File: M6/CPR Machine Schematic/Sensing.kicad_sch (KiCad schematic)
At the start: 14 parts, among them J6 I2C Port, J9 Force Sensor, U4 MCP6004, U5 MCP3021A5T-E_OT

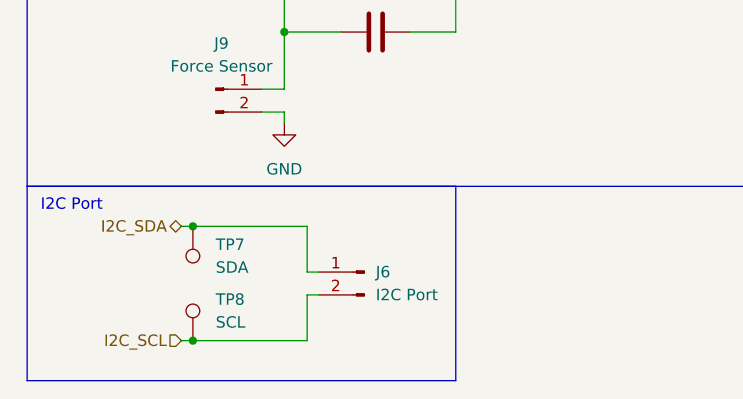
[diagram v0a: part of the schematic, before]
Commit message: More Revisions
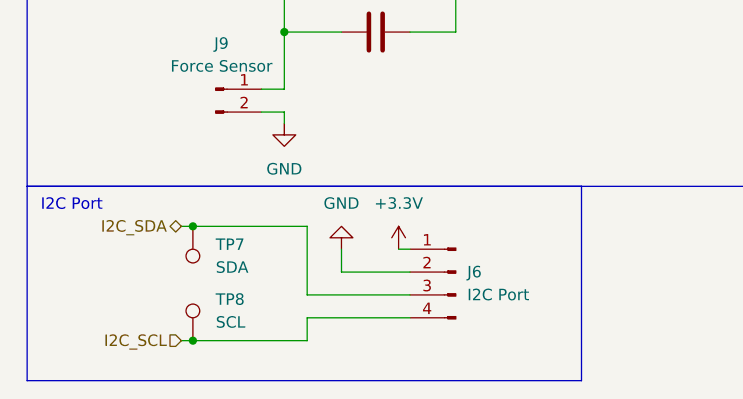
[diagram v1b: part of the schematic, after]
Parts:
- J6: footprint Connector_PinHeader_2.54mm:PinHeader_1x02_P2.54mm_Vertical -> Connector_PinHeader_2.54mm:PinHeader_1x04_P2.54mm_Vertical; symbol Connector:Conn_01x02_Pin -> Connector:Conn_01x04_Pin; now in the parts list
- U5: footprint 2679:IC_MCP3021A5T-E_OT -> 2679:IC_MCP3021A0T-E_OT
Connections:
- net +3.3V: now also J6.1 (Pin_1)
- net GND: now also J6.2 (Pin_2)
- net I2C_SCL: now also J6.4 (Pin_4); no longer J6.2 (Pin_2)
- net I2C_SDA: now also J6.3 (Pin_3); no longer J6.1 (Pin_1)
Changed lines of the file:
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@@
 	(rectangle
 		(start 14.605 84.455)
-		(end 62.23 106.045)
+		(end 76.2 106.045)
 		(stroke
 			(width 0)
@@
 	(wire
 		(pts
+			(xy 55.88 91.44) (xy 57.15 91.44)
+		)
+		(stroke
+			(width 0)
+			(type default)
+		)
+	)
+	(wire
+		(pts
 			(xy 33.02 101.6) (xy 31.75 101.6)
 		)
@@
 	(wire
 		(pts
-			(xy 45.72 93.98) (xy 46.99 93.98)
+			(xy 45.72 96.52) (xy 57.15 96.52)
+		)
+		(stroke
+			(width 0)
+			(type default)
+		)
+	)
+	(wire
+		(pts
+			(xy 49.53 91.44) (xy 49.53 93.98)
 		)
 		(stroke
@@
 	(wire
 		(pts
-			(xy 45.72 88.9) (xy 45.72 93.98)
+			(xy 45.72 88.9) (xy 45.72 96.52)
 		)
 		(stroke
@@
 	(wire
 		(pts
-			(xy 45.72 96.52) (xy 45.72 101.6)
+			(xy 45.72 99.06) (xy 45.72 101.6)
 		)
 		(stroke
@@
 	(wire
 		(pts
-			(xy 45.72 96.52) (xy 46.99 96.52)
+			(xy 45.72 99.06) (xy 57.15 99.06)
 		)
 		(stroke
@@
 		(pts
 			(xy 43.18 77.47) (xy 43.18 76.2)
+		)
+		(stroke
+			(width 0)
+			(type default)
+		)
+	)
+	(wire
+		(pts
+			(xy 49.53 93.98) (xy 57.15 93.98)
 		)
 		(stroke
@@
 	)
 	(symbol
-		(lib_id "Connector:Conn_01x02_Pin")
-		(at 52.07 93.98 0)
+		(lib_id "Connector:Conn_01x04_Pin")
+		(at 62.23 93.98 0)
 		(mirror y)
 		(unit 1)
 		(exclude_from_sim no)
-		(in_bom no)
+		(in_bom yes)
 		(on_board yes)
 		(dnp no)
 		(fields_autoplaced yes)
 		(property "Reference" "J6"
-			(at 53.34 93.9799 0)
+			(at 63.5 93.9799 0)
 			(effects
 				(font
@@
 		)
 		(property "Value" "I2C Port"
-			(at 53.34 96.5199 0)
+			(at 63.5 96.5199 0)
 			(effects
 				(font
@@
 			)
 		)
-		(property "Footprint" "Connector_PinHeader_2.54mm:PinHeader_1x02_P2.54mm_Vertical"
-			(at 52.07 93.98 0)
+		(property "Footprint" "Connector_PinHeader_2.54mm:PinHeader_1x04_P2.54mm_Vertical"
+			(at 62.23 93.98 0)
 			(effects
 				(font
@@
 		)
 		(property "Datasheet" "~"
-			(at 52.07 93.98 0)
-			(effects
-				(font
-					(size 1.27 1.27)
-				)
-				(hide yes)
-			)
-		)
-		(property "Description" "Generic connector, single row, 01x02, script generated"
-			(at 52.07 93.98 0)
+			(at 62.23 93.98 0)
+			(effects
+				(font
+					(size 1.27 1.27)
+				)
+				(hide yes)
+			)
+		)
+		(property "Description" "Generic connector, single row, 01x04, script generated"
+			(at 62.23 93.98 0)
 			(effects
 				(font
@@
 		)
 		(property "Notes" ""
-			(at 52.07 93.98 0)
+			(at 62.23 93.98 0)
 			(effects
 				(font
@@
 		)
 		(property "MPN" ""
-			(at 52.07 93.98 0)
+			(at 62.23 93.98 0)
 			(effects
 				(font
@@
 		)
 		(property "OC_FARNELL" ""
-			(at 52.07 93.98 0)
+			(at 62.23 93.98 0)
 			(effects
 				(font
@@
 		)
 		(property "OC_NEWARK" ""
-			(at 52.07 93.98 0)
+			(at 62.23 93.98 0)
 			(effects
 				(font
@@
 		)
 		(property "PACKAGE" ""
-			(at 52.07 93.98 0)
+			(at 62.23 93.98 0)
 			(effects
 				(font
@@
 		)
 		(property "SUPPLIER" ""
-			(at 52.07 93.98 0)
+			(at 62.23 93.98 0)
 			(effects
 				(font
@@
 		)
 		(pin "1"
+		)
+		(pin "3"
+		)
+		(pin "4"
 		)
 		(instances
@@
 			)
 		)
-		(property "Footprint" "2679:IC_MCP3021A5T-E_OT"
+		(property "Footprint" "2679:IC_MCP3021A0T-E_OT"
 			(at 82.55 35.56 0)
 			(effects
@@
 	)
 	(symbol
+		(lib_id "power:GND")
+		(at 49.53 91.44 180)
+		(unit 1)
+		(exclude_from_sim no)
+		(in_bom yes)
+		(on_board yes)
+		(dnp no)
+		(fields_autoplaced yes)
+		(property "Reference" "#PWR033"
+			(at 49.53 85.09 0)
+			(effects
+				(font
+					(size 1.27 1.27)
+				)
+				(hide yes)
+			)
+		)
+		(property "Value" "GND"
+			(at 49.53 86.36 0)
+			(effects
+				(font
+					(size 1.27 1.27)
+				)
+			)
+		)
+		(property "Footprint" ""
+			(at 49.53 91.44 0)
+			(effects
+				(font
+					(size 1.27 1.27)
+				)
+				(hide yes)
+			)
+		)
+		(property "Datasheet" ""
+			(at 49.53 91.44 0)
+			(effects
+				(font
+					(size 1.27 1.27)
+				)
+				(hide yes)
+			)
+		)
+		(property "Description" "Power symbol creates a global label with name \"GND\" , ground"
+			(at 49.53 91.44 0)
+			(effects
+				(font
+					(size 1.27 1.27)
+				)
+				(hide yes)
+			)
+		)
+		(pin "1"
+		)
+		(instances
+			(project ""
+				(path "/8991fc77-975f-4978-a089-6b2a5e33f59b/2e704a40-db78-4cf7-9f7e-cfc586f5aeb3"
+					(reference "#PWR033")
+					(unit 1)
+				)
+			)
+		)
+	)
+	(symbol
 		(lib_id "Device:C")
 		(at 110.49 41.91 180)
@@
 					(unit 1)
 				)
+			)
+		)
+	)
+	(symbol
+		(lib_id "power:+3.3V")
+		(at 55.88 91.44 0)
+		(unit 1)
+		(exclude_from_sim no)
+		(in_bom yes)
+		(on_board yes)
+		(dnp no)
+		(fields_autoplaced yes)
+		(property "Reference" "#PWR032"
+			(at 55.88 95.25 0)
+			(effects
+				(font
+					(size 1.27 1.27)
+				)
+				(hide yes)
+			)
+		)
+		(property "Value" "+3.3V"
+			(at 55.88 86.36 0)
+			(effects
+				(font
+					(size 1.27 1.27)
+				)
+			)
+		)
+		(property "Footprint" ""
+			(at 55.88 91.44 0)
+			(effects
+				(font
+					(size 1.27 1.27)
+				)
+				(hide yes)
+			)
+		)
+		(property "Datasheet" ""
+			(at 55.88 91.44 0)
+			(effects
+				(font
+					(size 1.27 1.27)
+				)
+				(hide yes)
+			)
+		)
+		(property "Description" "Power symbol creates a global label with name \"+3.3V\""
+			(at 55.88 91.44 0)
+			(effects
+				(font
+					(size 1.27 1.27)
+				)
+				(hide yes)
+			)
+		)
+		(pin "1"
+		)
+		(instances
+			(project ""
+				(path "/8991fc77-975f-4978-a089-6b2a5e33f59b/2e704a40-db78-4cf7-9f7e-cfc586f5aeb3"
+					(reference "#PWR032")
+					(unit 1)
+				)
